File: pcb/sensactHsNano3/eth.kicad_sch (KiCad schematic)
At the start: 29 parts, among them J4 HR911105A, U2 LAN8720A, X1 50MHz

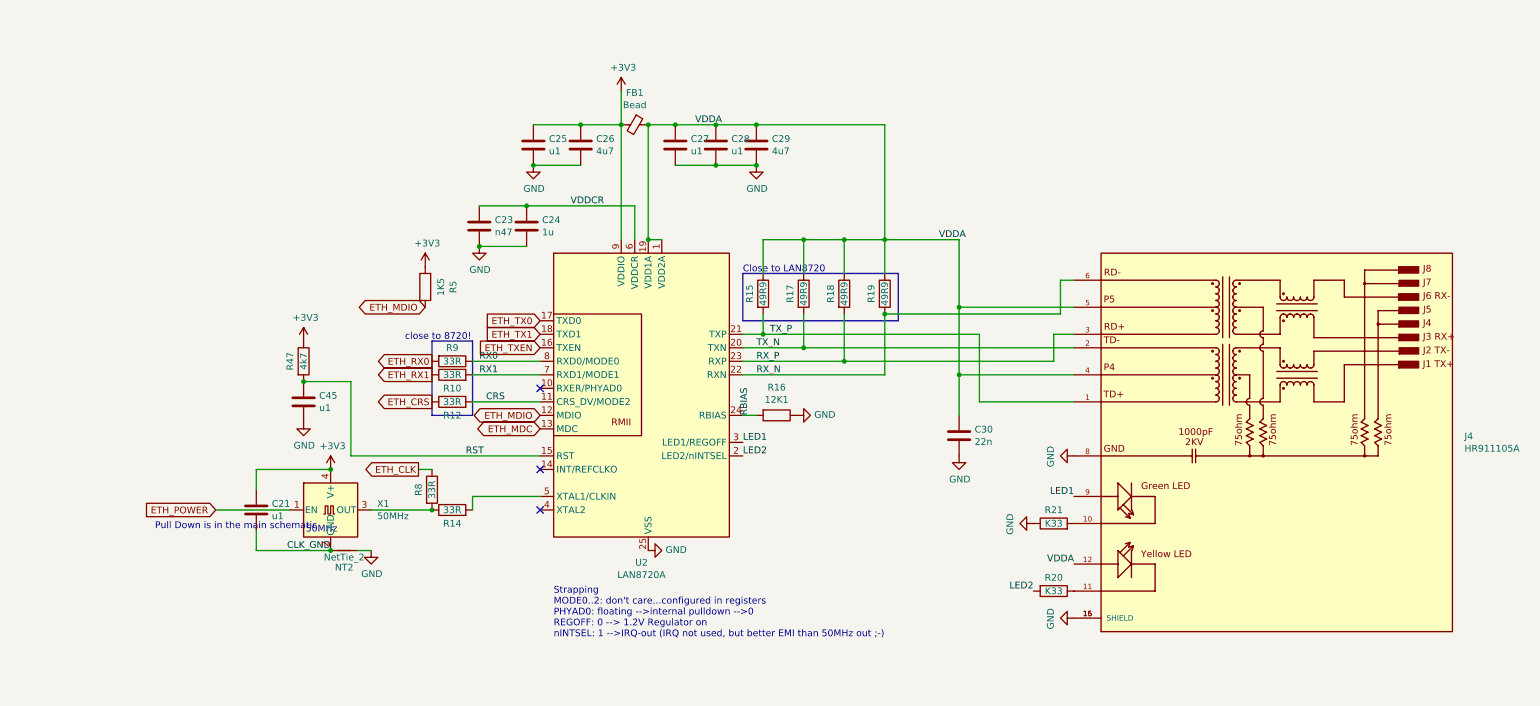
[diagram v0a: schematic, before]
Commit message: Updated various PCB
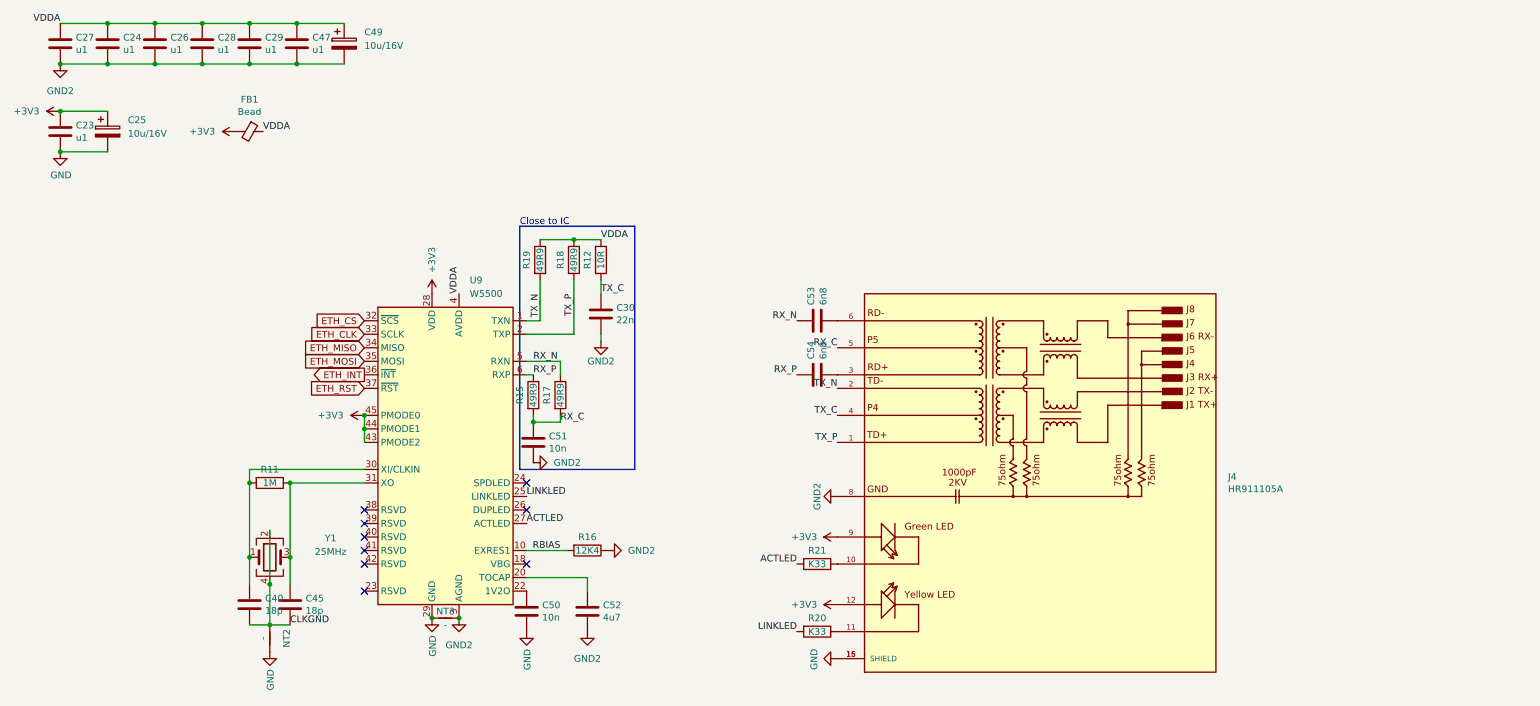
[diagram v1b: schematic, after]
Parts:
- removed C21, C25: u1, Capacitor_SMD:C_0402_1005Metric, symbol Device:C
- removed R10, R14, R8, R9: 33R, Resistor_SMD:R_0402_1005Metric, symbol Device:R
- removed R47: 4k7, Resistor_SMD:R_0402_1005Metric, symbol Device:R
- removed R5: 1K5, Resistor_SMD:R_0402_1005Metric, symbol Device:R
- removed U2: LAN8720A, Package_DFN_QFN:QFN-24-1EP_4x4mm_P0.5mm_EP2.6x2.6mm, symbol Interface_Ethernet:LAN8720A
- removed X1: 50MHz, Oscillator:Oscillator_SMD_SeikoEpson_SG8002CE-4Pin_3.2x2.5mm, symbol Oscillator:XO32
- added C25, C49: 10u/16V, Capacitor_Tantalum_SMD:CP_EIA-3216-18_Kemet-A, symbol Device:C_Polarized
- added C40: 18p, Capacitor_SMD:C_0402_1005Metric, symbol Device:C
- added C47: u1, Capacitor_SMD:C_0402_1005Metric, symbol Device:C
- added C50, C51: 10n, Capacitor_SMD:C_0402_1005Metric, symbol Device:C
- added C52: 4u7, Capacitor_SMD:C_0402_1005Metric, symbol Device:C
- added C53, C54: 6n8, Capacitor_SMD:C_0402_1005Metric, symbol Device:C
- added NT3: -, NetTie:NetTie-2_SMD_Pad0.5mm, symbol Device:NetTie_2
- added R11: 1M, Resistor_SMD:R_0402_1005Metric, symbol Device:R
- added U9: W5500, Package_QFP:LQFP-48_7x7mm_P0.5mm, symbol Interface_Ethernet:W5500
- added Y1: 25MHz, Crystal:Crystal_SMD_3225-4Pin_3.2x2.5mm, symbol Device:Crystal_GND24
- C23: value n47 -> u1
- C24: value 1u -> u1
- C26, C29: value 4u7 -> u1
- C30: footprint Capacitor_SMD:C_0805_2012Metric_Pad1.18x1.45mm_HandSolder -> Capacitor_SMD:C_0402_1005Metric
- C45: value u1 -> 18p
- FB1: footprint Inductor_SMD:L_0805_2012Metric_Pad1.15x1.40mm_HandSolder -> Inductor_SMD:L_0805_2012Metric
- NT2: value NetTie_2 -> -
- R12: value 33R -> 10R
- R16: value 12K1 -> 12K4
- R20, R21: footprint Resistor_SMD:R_0805_2012Metric_Pad1.20x1.40mm_HandSolder -> Resistor_SMD:R_0805_2012Metric
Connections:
- net CLK_GND is gone; now on net GND: NT2.1
- net ETH_CRS is gone; now on net VDDA: R12.1
- net LED1 is gone; now on net +3V3: J4.9
- net +3V3: now also C23.1, J4.12, C25.1, U9.28 (VDD), U9.43 (PMODE2), U9.44 (PMODE1), U9.45 (PMODE0); no longer C26.1
- net ETH_CLK: now also U9.33 (SCLK)
- net GND: now also C25.2, C50.2, NT3.2, U9.29 (GND); no longer C24.2, C26.2, C27.2, C28.2, C29.2, C30.2, C45.2, J4.8, NT2.2, R16.1, R21.1
- net RBIAS: now also U9.10 (EXRES1)
- net RX_N: now also R17.1, C53.1, U9.5 (RXN); no longer J4.6, R19.2
- net RX_P: now also R15.1, C54.1, U9.6 (RXP); no longer J4.3, R18.2
- net TX_N: now also R19.2, U9.1 (TXN); no longer R17.2
- net TX_P: now also R18.2, U9.2 (TXP); no longer R15.2
- net VDDA: now also C24.1, C26.1, C47.1, C49.1, U9.11 (AVDD), U9.15 (AVDD), U9.17 (AVDD), U9.21 (AVDD), U9.4 (AVDD), U9.8 (AVDD); no longer C30.1, J4.12, J4.4, J4.5, R15.1, R17.1
- net CRS renamed TX_C
- net TX_C: now also C30.1, J4.4
- net LED2 renamed LINKLED
- net LINKLED: now also U9.25 (LINKLED)
- net RST: no longer names the net of C45.1
- net RST: now also R11.1, U9.31 (XO), Y1.3
- removed net VDDCR: C23.1, C24.1
- new net: C54.2, J4.3
- new net: C53.2, J4.6
- new net: C40.1, R11.2, U9.30 (XI/CLKIN), Y1.1
- new net: C52.1, U9.20 (TOCAP)
- new net: C50.1, U9.22 (1V2O)
- new net ACTLED: R21.1, U9.27 (ACTLED)
- new net CLKGND: C40.2, C45.2, NT2.2, Y1.2, Y1.4
- new net ETH_CS: U9.32 (~{SCS})
- new net ETH_INT: U9.36 (~{INT})
- new net ETH_MISO: U9.34 (MISO)
- new net ETH_MOSI: U9.35 (MOSI)
- new net ETH_RST: U9.37 (~{RST})
- new net GND2: C24.2, C26.2, C27.2, C28.2, C29.2, C30.2, C47.2, C49.2, C51.2, C52.2, J4.8, NT3.1, R16.1, U9.14 (AGND), U9.16 (AGND), U9.19 (AGND), U9.3 (AGND), U9.48 (AGND), U9.9 (AGND)
- new net RX_C: C51.1, J4.5, R15.2, R17.2
- no-connect marks 3 -> 9
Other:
- note added: "Close to IC"
- note removed: "50MHz"
- note removed: "Close to LAN8720"
- note removed: "Pull Down is in the main schematic"
- note removed: "Strapping MODE0..2: don't care...configured in registers PHYAD0: floating -->internal pulldown -->0 REGOFF: 0 --> 1.2V Regulator on nINTSEL: 1 -->IRQ-out (IRQ not used, but better EMI than 50MHz out ;-)"
- note removed: "close to 8720!"
- moved on the sheet: C27, C30, FB1, J4, NT2, R15, R16, R17, R18, R19, R20, R21
